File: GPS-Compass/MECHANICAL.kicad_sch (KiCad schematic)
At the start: 16 parts, among them SW2 SW_Push, SW3 SW_Push, SW4 SW_Push, SW5 SW_Push

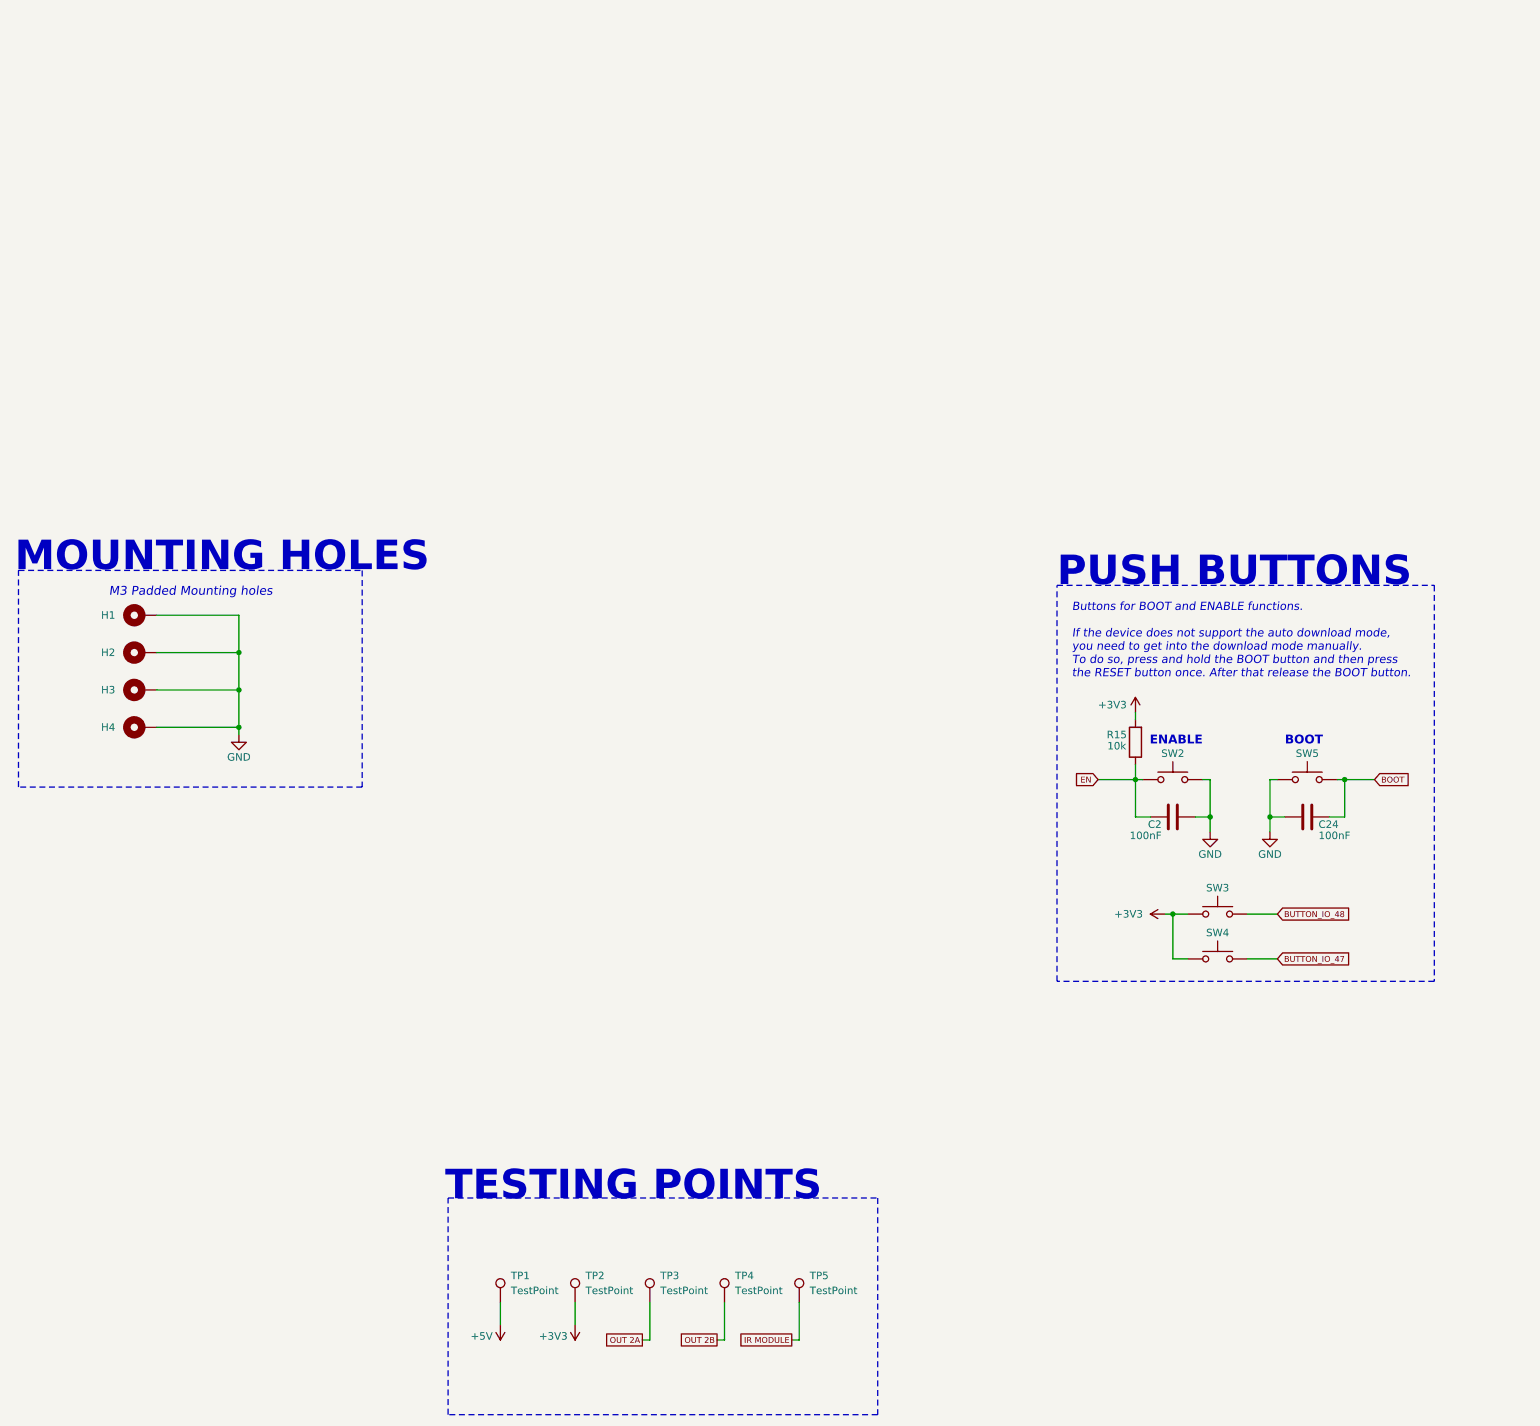
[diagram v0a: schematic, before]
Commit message: Schematic update
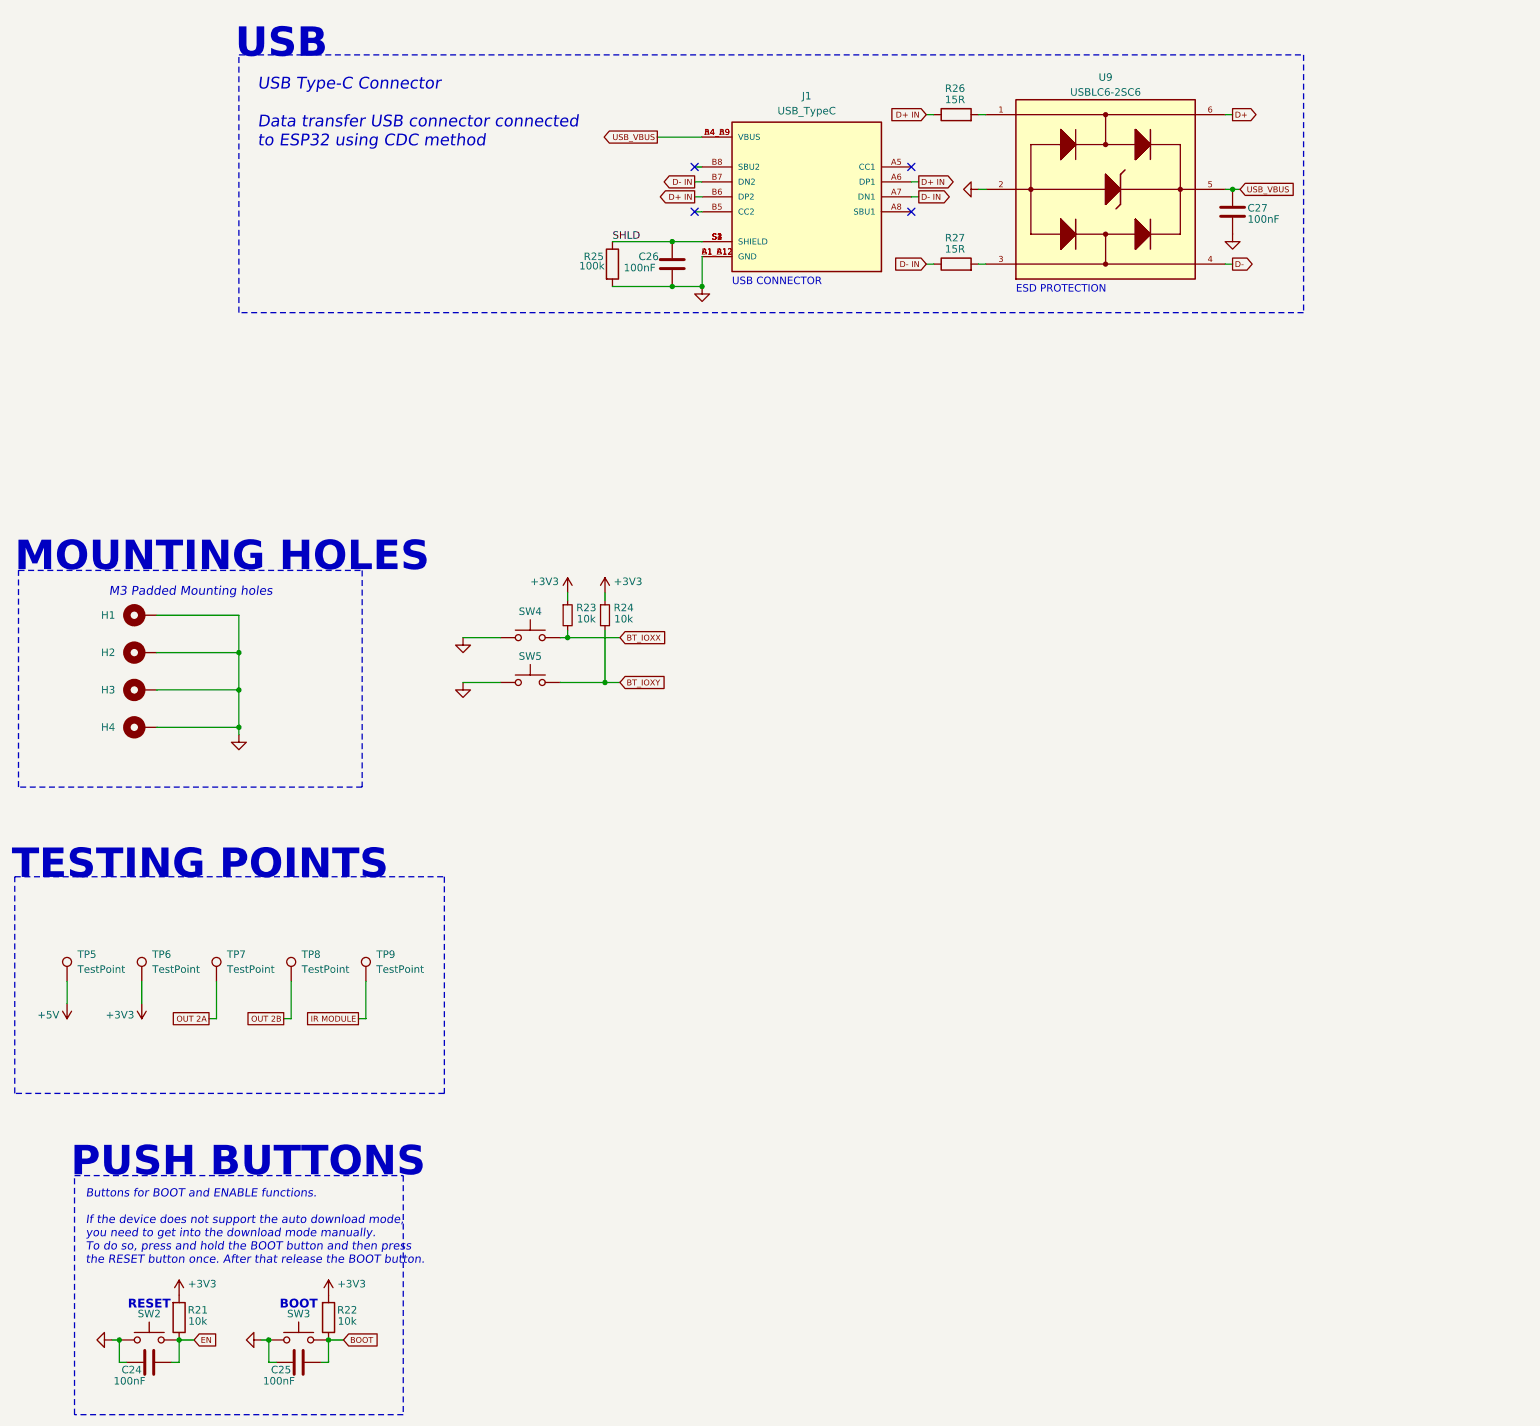
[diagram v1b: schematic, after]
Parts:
- removed C24: 100nF, Capacitor_SMD:C_0805_2012Metric_Pad1.18x1.45mm_HandSolder, symbol Device:C
- added C25, C26, C27: 100nF, Capacitor_SMD:C_0805_2012Metric_Pad1.18x1.45mm_HandSolder, symbol Device:C
- added J1: USB_TypeC, sumec_brd:HRO_TYPE-C-31-M-12, symbol sumec_sch_lib:USB_TypeC
- added R22: 10k, Resistor_SMD:R_0805_2012Metric_Pad1.20x1.40mm_HandSolder, symbol Device:R
- added R23, R24: 10k, symbol Device:R_Small
- added R25: 100k, Resistor_SMD:R_0805_2012Metric_Pad1.20x1.40mm_HandSolder, symbol Device:R
- added R26, R27: 15R, Resistor_SMD:R_0805_2012Metric_Pad1.20x1.40mm_HandSolder, symbol Device:R
- added U9: USBLC6-2SC6, Package_TO_SOT_SMD:TSOT-23-6_HandSoldering, symbol sumec_library:USBLC6-2SC6
- renumbered C2 to C24, R15 to R21, TP1 to TP5, TP2 to TP6, TP3 to TP7, TP4 to TP8, TP5 to TP9
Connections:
- net BUTTON_IO_48 is gone; now on net BOOT: SW3.2
- net +3V3: now also R22.2, R23.1, R24.1; no longer SW3.1, SW4.1
- net BOOT: now also C25.2, R22.1; no longer SW5.2
- net EN: now also C24.2; no longer C24.1
- net GND: now also C24.1, SW3.1, SW4.1, C25.1, C26.1, C27.2, J1.A1_B12 (GND), J1.B1_A12 (GND), R25.2, U9.2; no longer C24.2
- net BUTTON_IO_47 renamed BT_IOXX
- net BT_IOXX: now also R23.2
- new net: R26.2, U9.1
- new net: R27.2, U9.3
- new net BT_IOXY: R24.2, SW5.2
- new net D+: U9.6
- new net D+ IN: J1.A6 (DP1), J1.B6 (DP2), R26.1
- new net D-: U9.4
- new net D- IN: J1.A7 (DN1), J1.B7 (DN2), R27.1
- new net SHLD: C26.2, J1.S1 (SHIELD), J1.S2 (SHIELD), J1.S3 (SHIELD), J1.S4 (SHIELD), R25.1
- new net USB_VBUS: C27.1, J1.A4_B9 (VBUS), J1.B4_A9 (VBUS), U9.5
- no-connect marks 0 -> 4
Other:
- note added: "ESD PROTECTION"
- note added: "RESET"
- note added: "USB"
- note added: "USB CONNECTOR"
- note added: "USB Type-C Connector Data transfer USB connector connected to ESP32 using CDC method"
- note removed: "ENABLE"
- moved on the sheet: C24, R21, SW2, TP5, TP6, TP7, TP8, TP9
